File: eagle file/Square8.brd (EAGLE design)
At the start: 49.5 x 53 mm, 30 parts, among them J3 CR2032-172, Q1 si2305, U1 ATmega328mu, U2 CH340T, U3 CN3065, X1 16MHz, X2 12MHz

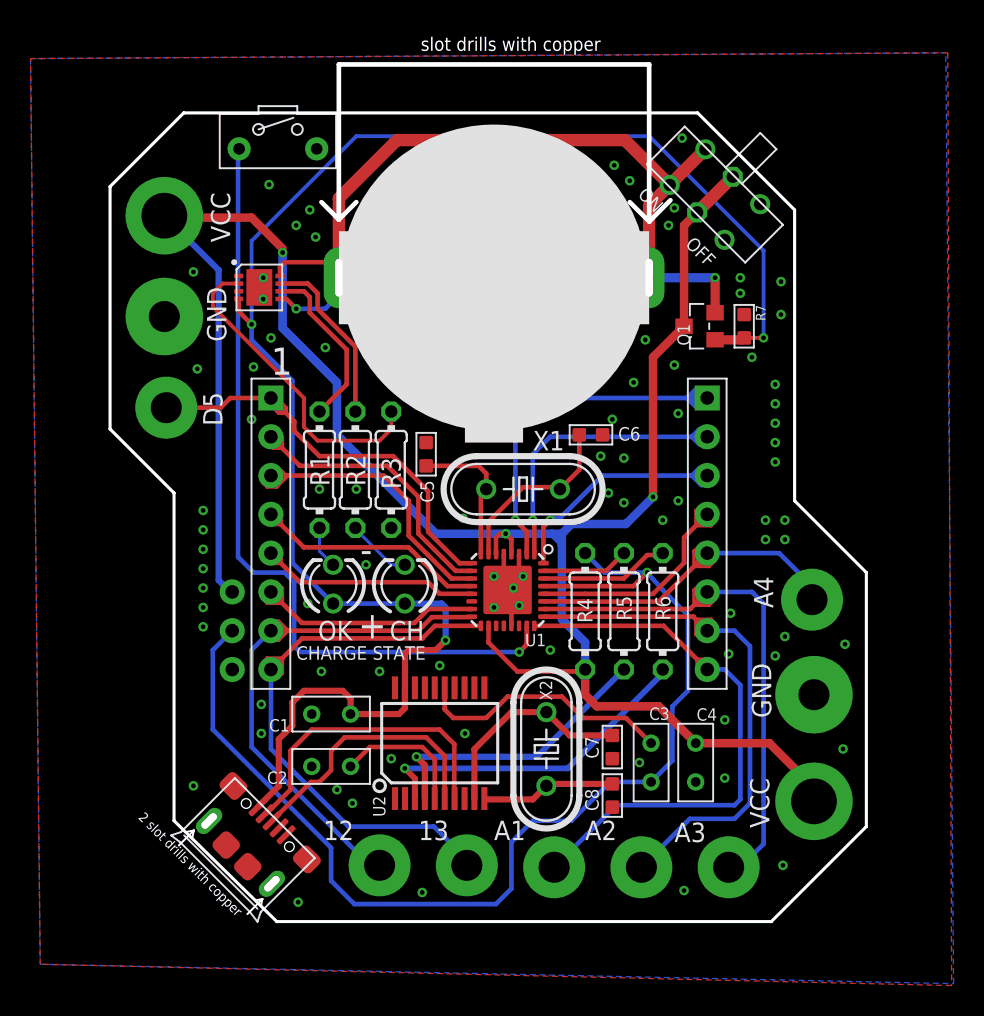
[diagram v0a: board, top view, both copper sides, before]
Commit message: improve pcb
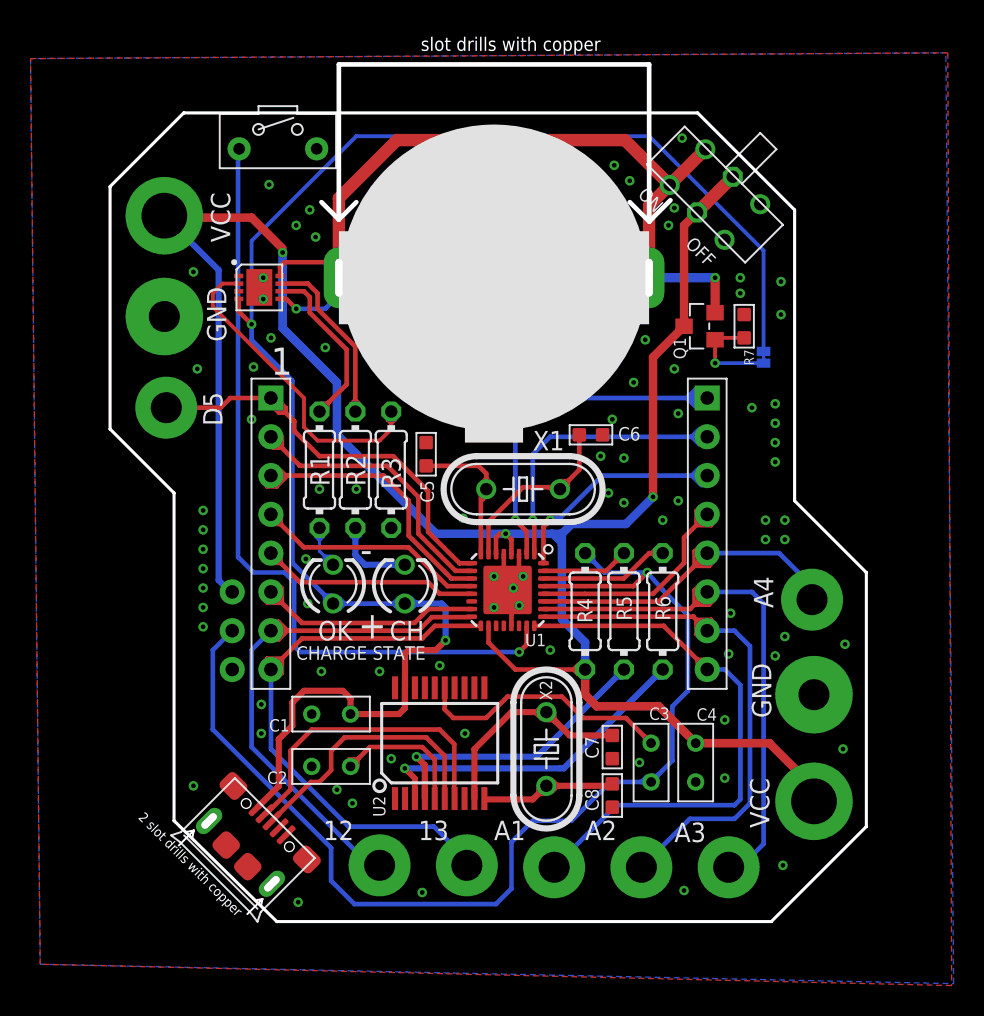
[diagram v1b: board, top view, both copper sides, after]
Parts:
- added P1: (no value), Discrete:2P-SMD-1.78X1.27
- moved U$1 0.09 mm to (30.9, 46.6)
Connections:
- new net N$86: P1.2, Q1.1, R7.2
- net USB5V: now also P1.1; no longer Q1.1, R7.2
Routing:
- net N$86: track 0.00 -> 6.66 mm, vias 0 -> 1
- net N$4: track 2.78 -> 4.77 mm
- net XTAL1: track 11.9 -> 13.8 mm
- net N$5: track 4.28 -> 5.95 mm
- net N$40: track 8.82 -> 9.99 mm
- net V3: track 8.93 -> 10.1 mm
- net RESET: track 74.3 -> 75.3 mm
- net N$7: track 20.7 -> 21.6 mm
- net PD0/RX: track 8.50 -> 9.40 mm
- net N$3: track 11.3 -> 12.2 mm
- net N$100: track 0.00 -> 0.73 mm
- net XTAL2: track 9.61 -> 10.3 mm
- net N$110: track 0.00 -> 0.70 mm
- net N$111: track 0.00 -> 0.67 mm
- net N$39: track 13.9 -> 14.5 mm
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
